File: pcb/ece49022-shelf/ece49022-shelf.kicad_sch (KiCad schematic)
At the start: 9 parts, among them J2 Conn_01x16_Pin, J3 Conn_01x04_Pin, J6 Conn_01x02_Pin, J7 Conn_01x02_Pin

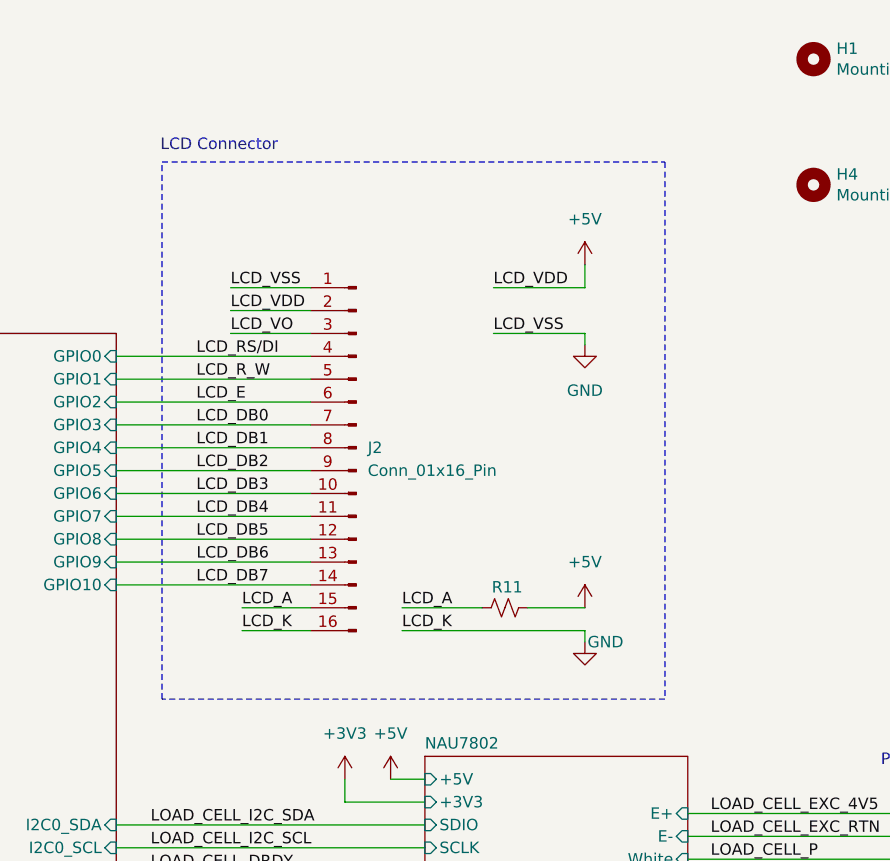
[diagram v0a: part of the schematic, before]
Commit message: working on stuff
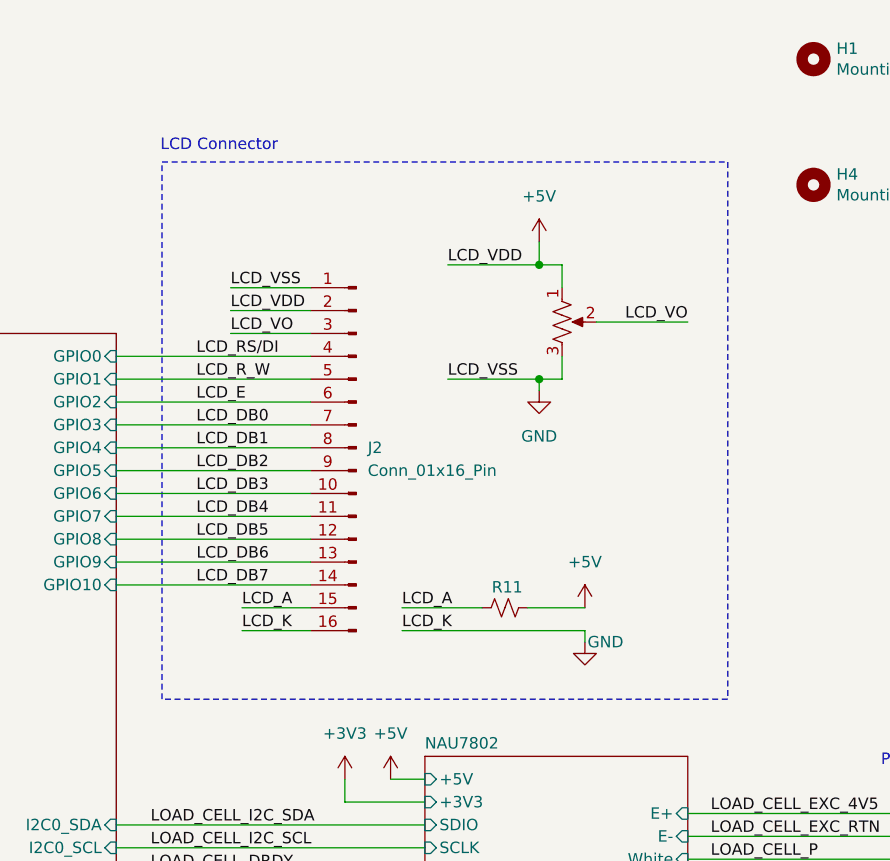
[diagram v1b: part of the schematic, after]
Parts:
- added RV1: R_Potentiometer_US, 49022_Footprints:RES_C01R00, symbol Device:R_Potentiometer_US
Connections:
- net +5V: now also RV1.1
- net GND: now also RV1.3
- net LCD_VO: now also RV1.2
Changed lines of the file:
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@@
 	(rectangle
 		(start 140.97 55.88)
-		(end 196.85 115.57)
+		(end 203.835 115.57)
 		(stroke
 			(width 0)
@@
 		)
 	)
+	(junction
+		(at 182.88 80.01)
+		(diameter 0)
+		(color 0 0 0 0)
+	)
+	(junction
+		(at 182.88 67.31)
+		(diameter 0)
+		(color 0 0 0 0)
+	)
 	(wire
 		(pts
@@
 	(wire
 		(pts
+			(xy 182.88 67.31) (xy 185.42 67.31)
+		)
+		(stroke
+			(width 0)
+			(type default)
+		)
+	)
+	(wire
+		(pts
 			(xy 135.89 132.08) (xy 170.18 132.08)
 		)
@@
 	(wire
 		(pts
+			(xy 185.42 77.47) (xy 185.42 80.01)
+		)
+		(stroke
+			(width 0)
+			(type default)
+		)
+	)
+	(wire
+		(pts
 			(xy 90.17 81.28) (xy 90.17 83.82)
 		)
@@
 	(wire
 		(pts
-			(xy 187.96 74.93) (xy 187.96 76.2)
+			(xy 182.88 80.01) (xy 182.88 81.28)
 		)
 		(stroke
@@
 	(wire
 		(pts
+			(xy 185.42 67.31) (xy 185.42 69.85)
+		)
+		(stroke
+			(width 0)
+			(type default)
+		)
+	)
+	(wire
+		(pts
 			(xy 99.06 40.64) (xy 99.06 41.91)
 		)
@@
 	(wire
 		(pts
-			(xy 177.8 69.85) (xy 187.96 69.85)
+			(xy 172.72 67.31) (xy 182.88 67.31)
 		)
 		(stroke
@@
 	(wire
 		(pts
-			(xy 187.96 67.31) (xy 187.96 69.85)
+			(xy 182.88 64.77) (xy 182.88 67.31)
 		)
 		(stroke
@@
 	(wire
 		(pts
+			(xy 189.23 73.66) (xy 199.39 73.66)
+		)
+		(stroke
+			(width 0)
+			(type default)
+		)
+	)
+	(wire
+		(pts
 			(xy 181.61 105.41) (xy 187.96 105.41)
 		)
@@
 	(wire
 		(pts
+			(xy 182.88 80.01) (xy 185.42 80.01)
+		)
+		(stroke
+			(width 0)
+			(type default)
+		)
+	)
+	(wire
+		(pts
 			(xy 48.26 118.11) (xy 48.26 119.38)
 		)
@@
 	(wire
 		(pts
-			(xy 177.8 74.93) (xy 187.96 74.93)
+			(xy 172.72 80.01) (xy 182.88 80.01)
 		)
 		(stroke
@@
 	)
 	(label "LCD_VSS"
-		(at 177.8 74.93 0)
+		(at 172.72 80.01 0)
 		(effects
 			(font
@@
 	)
 	(label "LCD_VDD"
-		(at 177.8 69.85 0)
+		(at 172.72 67.31 0)
 		(effects
 			(font
@@
 			)
 			(justify left bottom)
+		)
+	)
+	(label "LCD_VO"
+		(at 199.39 73.66 180)
+		(effects
+			(font
+				(size 1.27 1.27)
+			)
+			(justify right bottom)
 		)
 	)
@@
 	)
 	(symbol
+		(lib_id "Device:R_Potentiometer_US")
+		(at 185.42 73.66 0)
+		(unit 1)
+		(exclude_from_sim no)
+		(in_bom yes)
+		(on_board yes)
+		(dnp no)
+		(fields_autoplaced yes)
+		(property "Reference" "RV1"
+			(at 182.88 72.3899 0)
+			(effects
+				(font
+					(size 1.27 1.27)
+				)
+				(justify right)
+				(hide yes)
+			)
+		)
+		(property "Value" "R_Potentiometer_US"
+			(at 182.88 74.9299 0)
+			(effects
+				(font
+					(size 1.27 1.27)
+				)
+				(justify right)
+				(hide yes)
+			)
+		)
+		(property "Footprint" "49022_Footprints:RES_C01R00"
+			(at 185.42 73.66 0)
+			(effects
+				(font
+					(size 1.27 1.27)
+				)
+				(hide yes)
+			)
+		)
+		(property "Datasheet" "~"
+			(at 185.42 73.66 0)
+			(effects
+				(font
+					(size 1.27 1.27)
+				)
+				(hide yes)
+			)
+		)
+		(property "Description" "Potentiometer, US symbol"
+			(at 185.42 73.66 0)
+			(effects
+				(font
+					(size 1.27 1.27)
+				)
+				(hide yes)
+			)
+		)
+		(pin "3"
+		)
+		(pin "1"
+		)
+		(pin "2"
+		)
+		(instances
+			(project ""
+				(path "/cb6cb1b4-c151-4aa2-8cd7-5430288cfa02"
+					(reference "RV1")
+					(unit 1)
+				)
+			)
+		)
+	)
+	(symbol
 		(lib_id "power:+5V")
 		(at 105.41 40.64 0)
@@
 	(symbol
 		(lib_id "power:GND")
-		(at 187.96 76.2 0)
+		(at 182.88 81.28 0)
 		(unit 1)
 		(exclude_from_sim no)
@@
 		(fields_autoplaced yes)
 		(property "Reference" "#PWR049"
-			(at 187.96 82.55 0)
+			(at 182.88 87.63 0)
 			(effects
 				(font
@@
 		)
 		(property "Value" "GND"
-			(at 187.96 81.28 0)
+			(at 182.88 86.36 0)
 			(effects
 				(font
@@
 		)
 		(property "Footprint" ""
-			(at 187.96 76.2 0)
+			(at 182.88 81.28 0)
 			(effects
 				(font
@@
 		)
 		(property "Datasheet" ""
-			(at 187.96 76.2 0)
+			(at 182.88 81.28 0)
 			(effects
 				(font
@@
 		)
 		(property "Description" "Power symbol creates a global label with name \"GND\" , ground"
-			(at 187.96 76.2 0)
+			(at 182.88 81.28 0)
 			(effects
 				(font
@@
 	(symbol
 		(lib_id "power:+5V")
-		(at 187.96 67.31 0)
+		(at 182.88 64.77 0)
 		(unit 1)
 		(exclude_from_sim no)
@@
 		(fields_autoplaced yes)
 		(property "Reference" "#PWR050"
-			(at 187.96 71.12 0)
+			(at 182.88 68.58 0)
 			(effects
 				(font
@@
 		)
 		(property "Value" "+5V"
-			(at 187.96 62.23 0)
+			(at 182.88 59.69 0)
 			(effects
 				(font
@@
 		)
 		(property "Footprint" ""
-			(at 187.96 67.31 0)
+			(at 182.88 64.77 0)
 			(effects
 				(font
@@
 		)
 		(property "Datasheet" ""
-			(at 187.96 67.31 0)
+			(at 182.88 64.77 0)
 			(effects
 				(font
@@
 		)
 		(property "Description" "Power symbol creates a global label with name \"+5V\""
-			(at 187.96 67.31 0)
-			(effects
-				(font
+			(at 182.88 64.77 0)
+			(effects
+				(font
